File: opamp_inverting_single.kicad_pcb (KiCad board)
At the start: 2 copper layers, 17 parts, among them J1 Conn_Coaxial, J2 Conn_Coaxial, J3 Power-NanoFit-01x03, U1 LT1722xS8

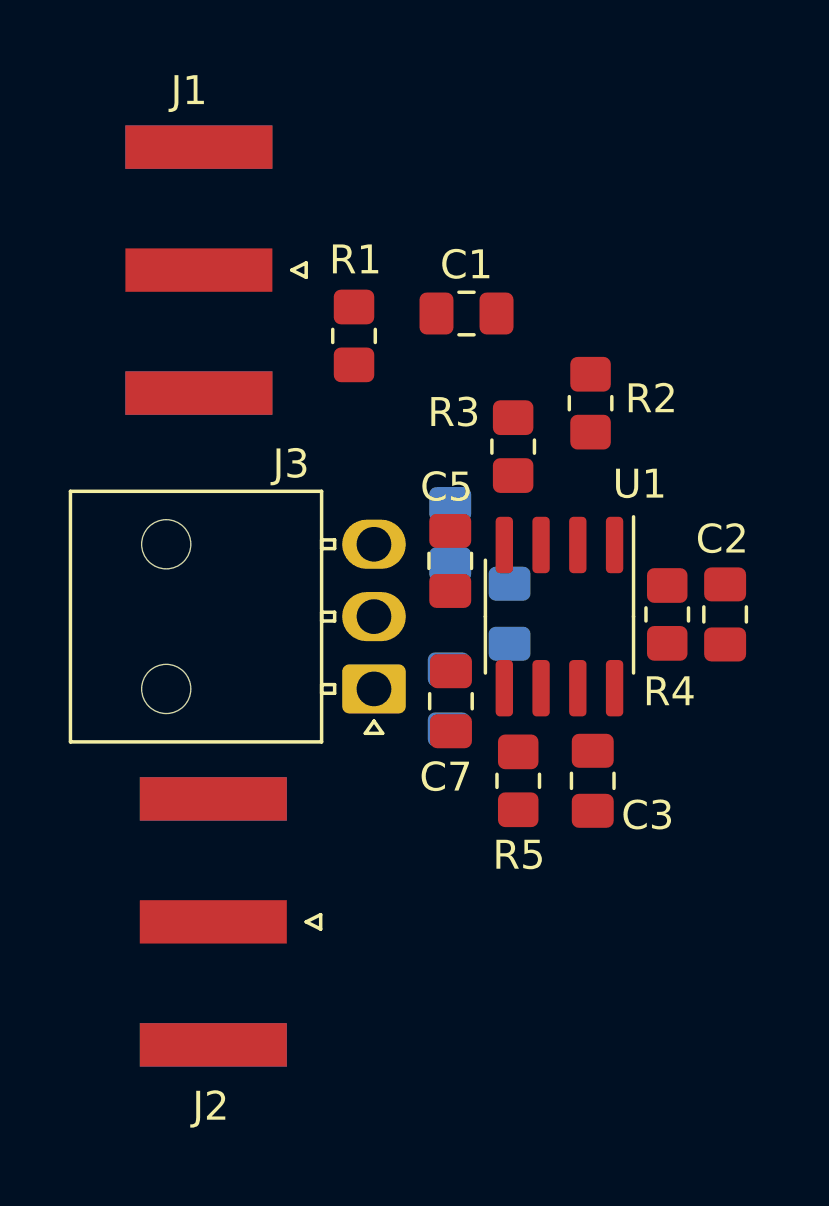
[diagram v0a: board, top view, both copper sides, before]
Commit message: some routing
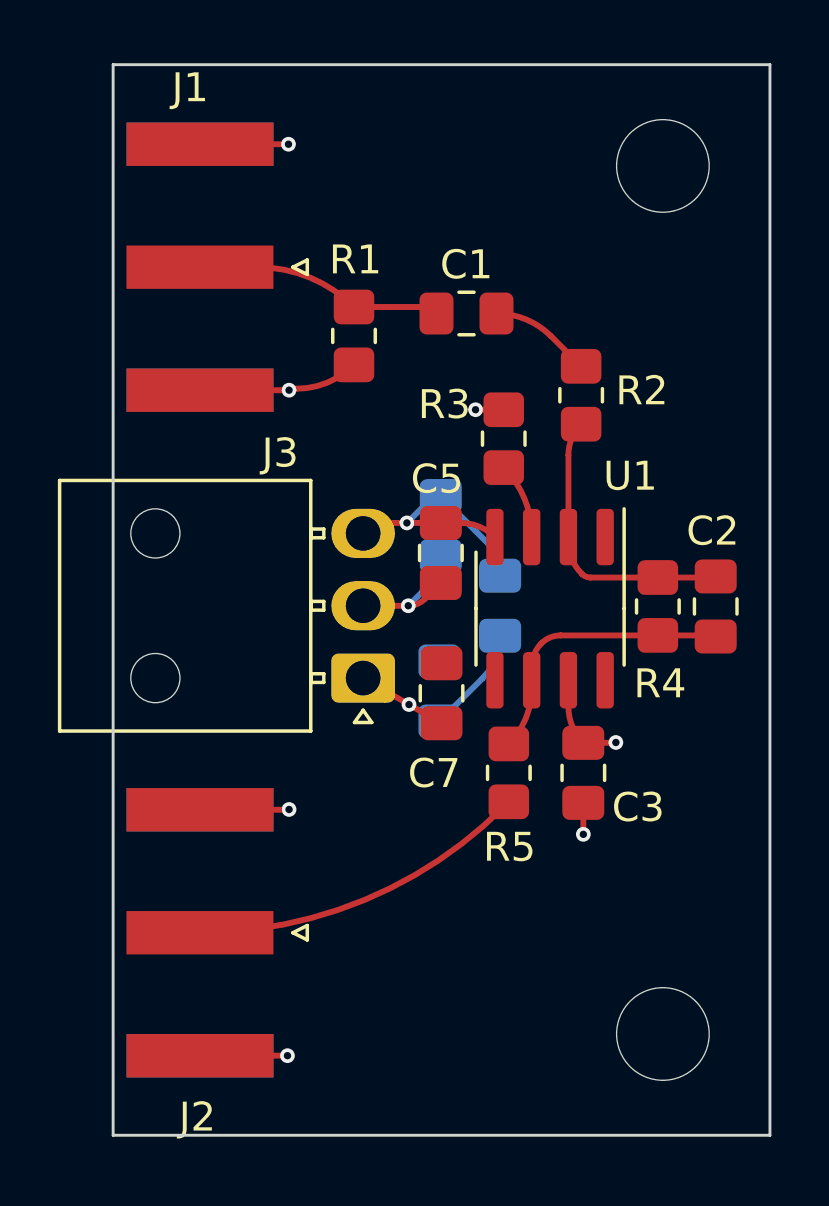
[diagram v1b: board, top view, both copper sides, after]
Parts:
- added REF**: MountingHole_3.2mm_M3, MountingHole:MountingHole_3.2mm_M3, F.Cu at (160.8, 72.3)
- added REF**: MountingHole_3.2mm_M3, MountingHole:MountingHole_3.2mm_M3, F.Cu at (160.8, 102.3)
- moved J2 0.60 mm to (144.8, 98.8)
- moved J3 0.53 mm to (150.5, 90.0)
- moved C8 0.43 mm to (155.2, 87.5)
- moved R3 0.43 mm to (155.3, 81.7)
- moved C3 0.43 mm to (158.1, 93.3)
- moved C4 0.43 mm to (153.1, 90.5)
- moved C5 0.43 mm to (153.1, 85.7)
- moved C6 0.43 mm to (153.1, 84.7)
- moved R2 0.43 mm to (158.0, 80.2)
- moved U1 0.43 mm to (156.9, 87.6)
- moved C2 0.43 mm to (162.6, 87.5)
- moved C7 0.43 mm to (153.2, 90.5), turned to -90 degrees
- moved R4 0.43 mm to (160.6, 87.5)
- moved R5 0.43 mm to (155.5, 93.3)
- moved J1 0.11 mm to (144.8, 75.8)
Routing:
- net GND: track 0.00 -> 21.9 mm, vias 0 -> 7
- net /coax_out: track 0.00 -> 12.1 mm
- net +5V: track 0.00 -> 11.3 mm, vias 0 -> 2
- net /inv_in: track 0.00 -> 10.1 mm
- net /amp_out: track 0.00 -> 9.86 mm
- net -5V: track 0.00 -> 9.81 mm, vias 0 -> 1
- net /coax_in: track 0.00 -> 8.58 mm
- net /Cblock_Rin: track 0.00 -> 3.55 mm
- net /non_inv_in: track 0.00 -> 2.64 mm
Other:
- board outline added: 22.7 x 37 mm
- board text added: "2x M3 screw holes"
